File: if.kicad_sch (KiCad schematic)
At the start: 63 parts, among them U2 SolderPad_1_Circle, U31 SolderPad_1_Circle, U34 ADA4940-2, U35 ADA4940-2, U37 SolderPad_1_Circle, U5 SolderPad_1_Circle

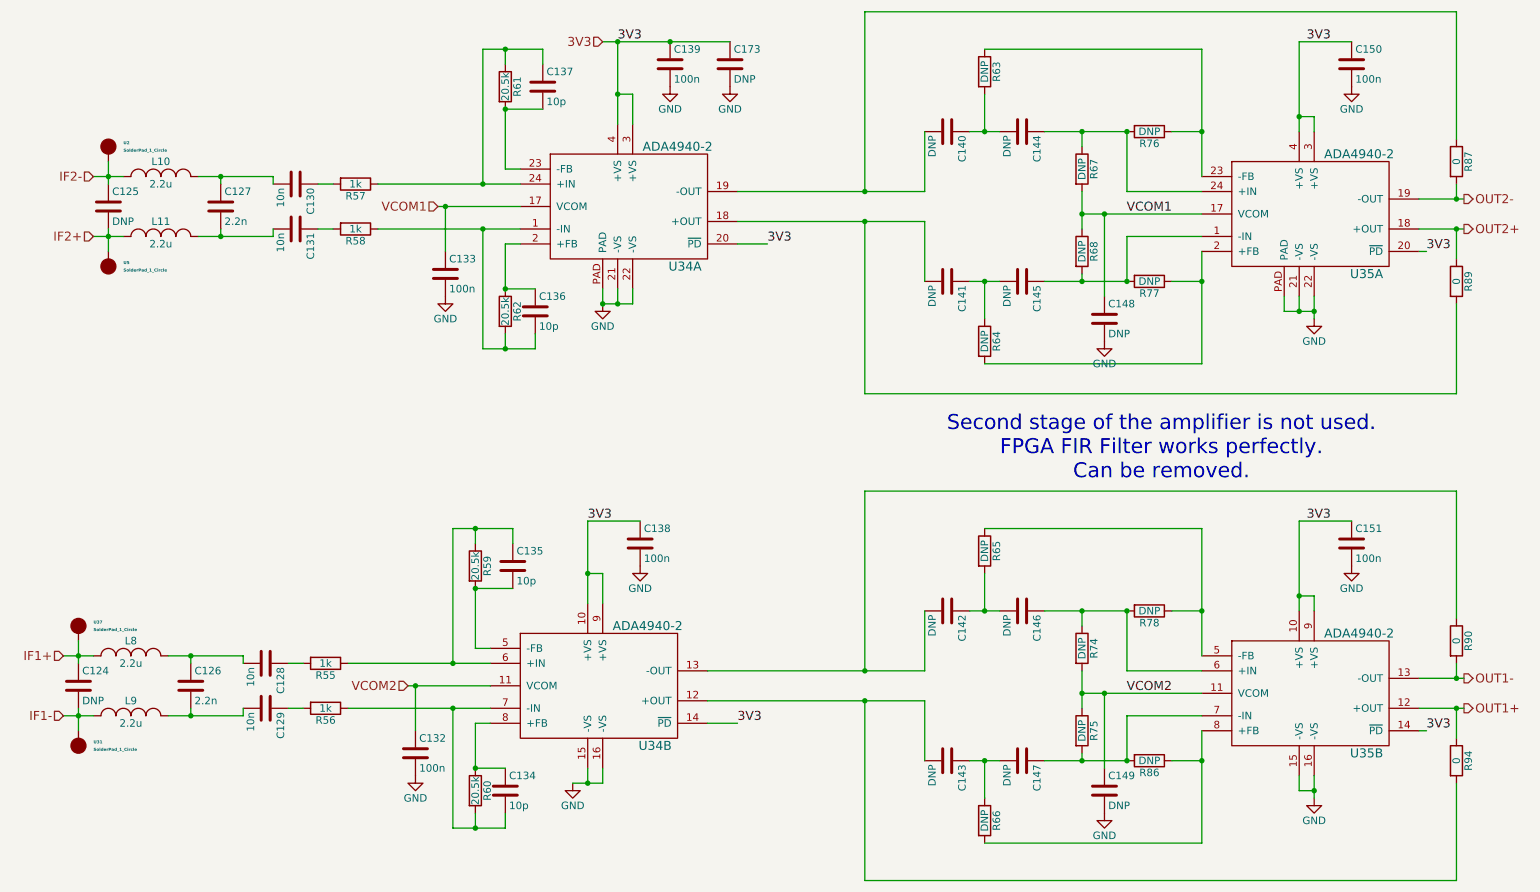
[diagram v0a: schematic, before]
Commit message: hardware changes
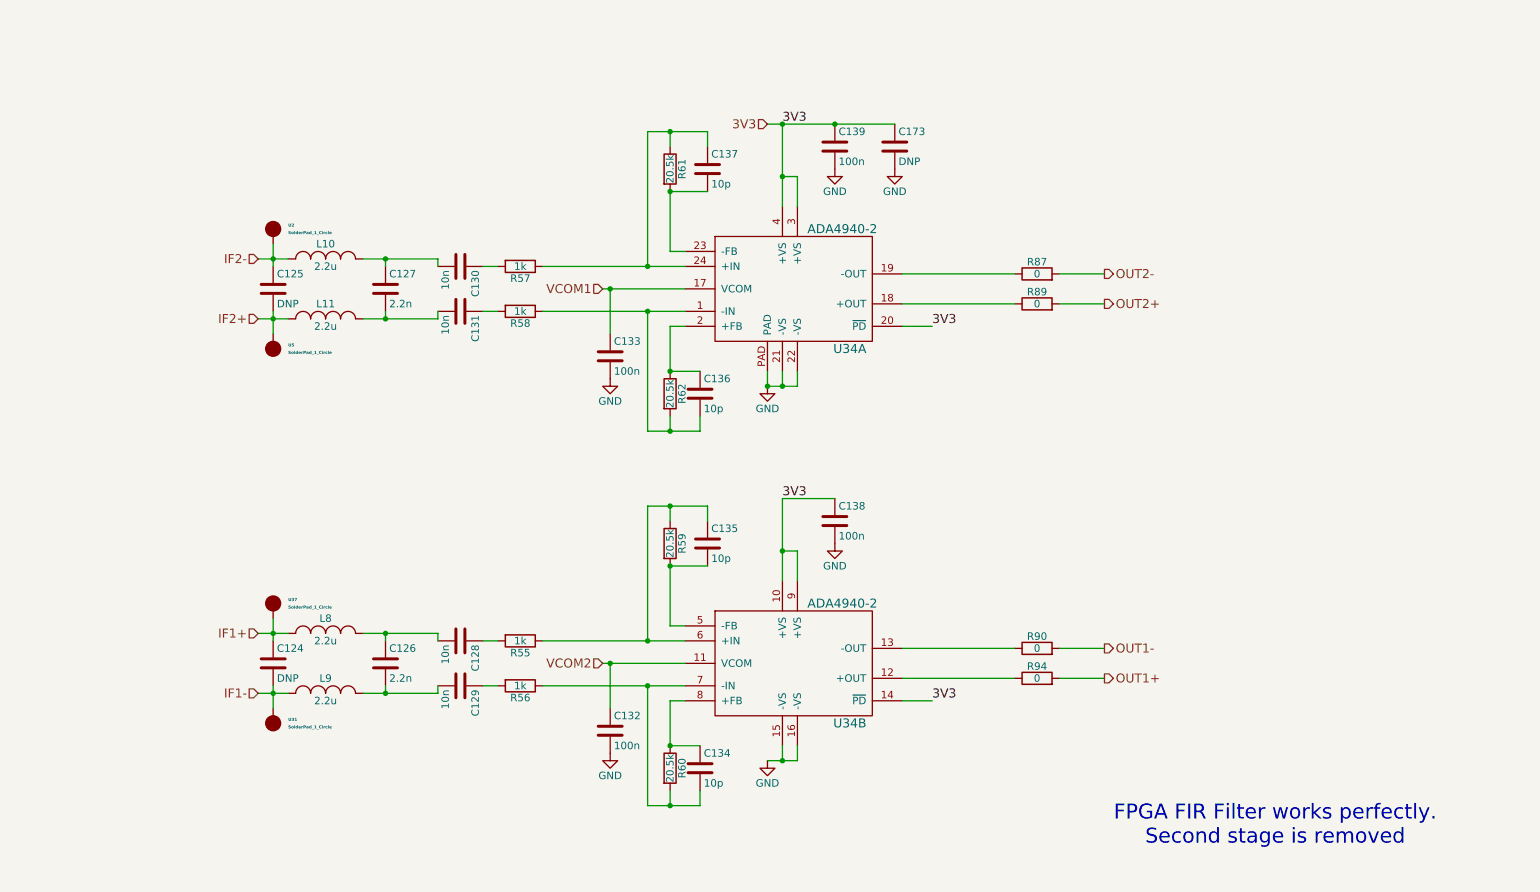
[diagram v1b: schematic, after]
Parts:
- removed C140, C141, C142, C143, C144, C145, C146, C147, C148, C149: DNP, Footprints:SMD_0402, symbol fmcw3-rescue:C
- removed C150, C151: 100n, Footprints:SMD_0402, symbol fmcw3-rescue:C
- removed R63, R64, R65, R66, R67, R68, R74, R75, R76, R77, R78, R86: DNP, Footprints:SMD_0402, symbol fmcw3-rescue:R
- removed U35: ADA4940-2, fmcw3:VFQFN-24, symbol fmcw3:ADA4940-2
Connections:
- net OUT1+: now also R94.2; no longer R94.1
- net OUT2+: now also R89.2; no longer R89.1
- net at U34.18 (+OUT): now also R89.1; no longer R89.2
- net at U34.12 (+OUT): now also R94.1; no longer R94.2
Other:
- note added: "FPGA FIR Filter works perfectly. Second stage is removed"
- note removed: "Second stage of the amplifier is not used. FPGA FIR Filter works perfectly. Can be removed."
- moved on the sheet: C124, C125, C126, C127, C128, C129, C130, C131, C132, C133, C134, C135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
